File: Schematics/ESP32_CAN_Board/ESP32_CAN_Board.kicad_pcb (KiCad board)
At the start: 2 copper layers, 23 parts, among them J8 USB_C_Receptacle, U1 SN65HVD230, U7 LDL1117-3.3

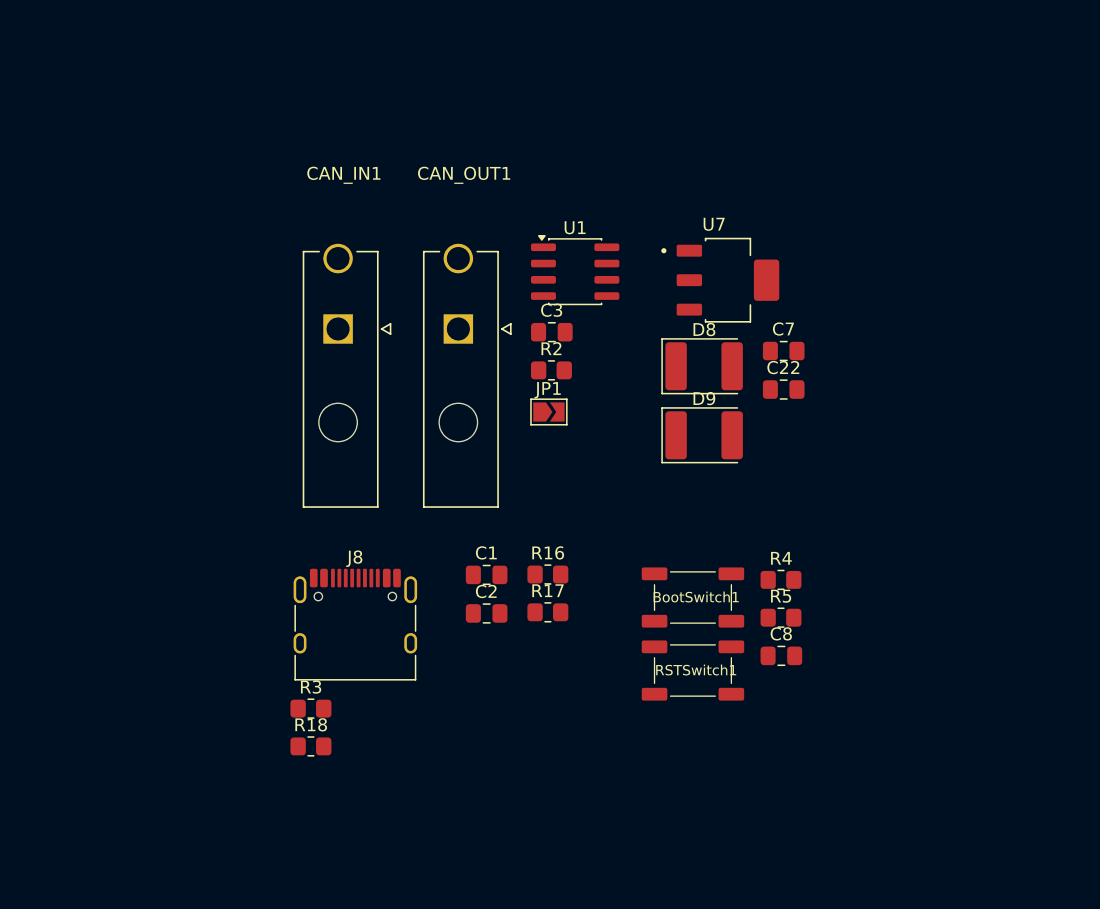
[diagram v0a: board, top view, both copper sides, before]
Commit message: initial design completed
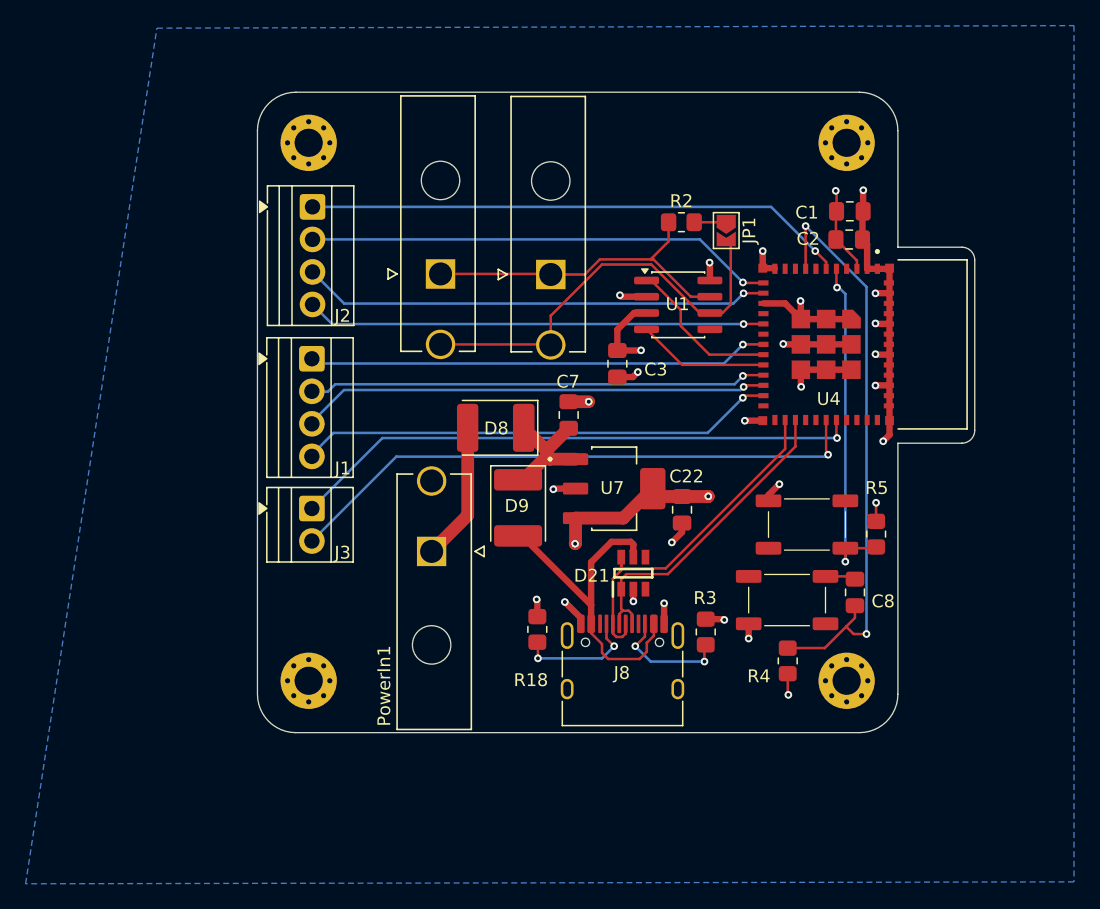
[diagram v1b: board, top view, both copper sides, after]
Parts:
- removed R16, R17: 10k, Resistor_SMD:R_0805_2012Metric_Pad1.20x1.40mm_HandSolder
- added D21: SRV05-4.TCT, myFootprints:SOT95P280X145-6N, F.Cu at (129.3, 87.5)
- added J1: Screw_Terminal_01x04, TerminalBlock:TerminalBlock_Xinya_XY308-2.54-4P_1x04_P2.54mm_Horizontal, F.Cu at (104.2, 70.8)
- added J2: Screw_Terminal_01x04, TerminalBlock:TerminalBlock_Xinya_XY308-2.54-4P_1x04_P2.54mm_Horizontal, F.Cu at (104.3, 59.0)
- added J3: Screw_Terminal_01x02, TerminalBlock:TerminalBlock_Xinya_XY308-2.54-2P_1x02_P2.54mm_Horizontal, F.Cu at (104.2, 82.5)
- added PowerIn1: 2 pin Molex, myFootprints:MOLEX_26013114, F.Cu at (113.6, 85.8)
- added REF**: MountingHole_2.2mm_M2_Pad_Via, MountingHole:MountingHole_2.2mm_M2_Pad_Via, F.Cu at (146.0, 96.0)
- added REF**: MountingHole_2.2mm_M2_Pad_Via, MountingHole:MountingHole_2.2mm_M2_Pad_Via, F.Cu at (104.0, 96.0)
- added REF**: MountingHole_2.2mm_M2_Pad_Via, MountingHole:MountingHole_2.2mm_M2_Pad_Via, F.Cu at (146.0, 54.0)
- added REF**: MountingHole_2.2mm_M2_Pad_Via, MountingHole:MountingHole_2.2mm_M2_Pad_Via, F.Cu at (104.0, 54.0)
- added U4: ESP32-C3-MINI-1-N4, myFootprints:XCVR_ESP32-C3-MINI-1-N4, F.Cu at (147.1, 69.7)
- moved C2 40.7 mm to (146.2, 61.5)
- moved C1 40.1 mm to (146.2, 59.3)
- moved R3 31.4 mm to (135.0, 92.1), turned to 90 degrees
- moved J8 21.2 mm to (128.5, 95.5)
- moved R18 19.9 mm to (121.8, 91.9), turned to 90 degrees
- moved JP1 19.8 mm to (136.6, 60.8), turned to -90 degrees
- moved U7 18.5 mm to (127.8, 81.0)
- moved C7 17.5 mm to (124.3, 75.2), turned to 90 degrees
- moved D8 17.0 mm to (118.6, 76.2), turned to 180 degrees
- moved D9 15.6 mm to (120.3, 82.5), turned to -90 degrees
- moved R2 15.4 mm to (133.1, 60.1)
- moved C22 12.3 mm to (133.2, 82.6), turned to -90 degrees
- moved BootSwitch1 10.6 mm to (142.9, 83.8)
- moved R5 9.88 mm to (148.3, 84.5), turned to -90 degrees
- moved RSTSwitch1 9.18 mm to (141.3, 89.7)
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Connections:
- C1 pad 1: /MCU/ESPPower -> +3.3V
- C2 pad 1: /MCU/ESPPower -> +3.3V
- C22 pad 1: /MCU/ESPPower -> +3.3V
- U7 pad 3: /MCU/ESPPower -> +3.3V
- U7 pad 4: /MCU/ESPPower -> +3.3V
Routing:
- net GND: track 0.00 -> 69.9 mm, vias 0 -> 24
- net /MCU/NRST: track 0.00 -> 46.2 mm, vias 0 -> 2
- net Net-(J3-Pin_2): track 0.00 -> 45.9 mm, vias 0 -> 1
- net Net-(J3-Pin_1): track 0.00 -> 44.7 mm, vias 0 -> 1
- net /MCU/Pin6: track 0.00 -> 42.4 mm, vias 0 -> 1
- net Net-(J1-Pin_4): track 0.00 -> 37.4 mm, vias 0 -> 1
- net Net-(J1-Pin_3): track 0.00 -> 36.7 mm, vias 0 -> 1
- net /MCU/Pin12: track 0.00 -> 36.6 mm, vias 0 -> 1
- net /MCU/Pin13: track 0.00 -> 36.6 mm, vias 0 -> 1
- net /MCU/Pin18: track 0.00 -> 36.2 mm, vias 0 -> 1
- net Net-(J1-Pin_2): track 0.00 -> 36.0 mm, vias 0 -> 1
- net /MCU/Pin16: track 0.00 -> 35.8 mm, vias 0 -> 1
- net /CAN/CANL: track 0.00 -> 33.7 mm
- net +3.3V: track 0.00 -> 29.0 mm, vias 0 -> 6
- net /MCU/D-: track 0.00 -> 28.0 mm
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- added copper zone on In2.Cu, net +3.3V
- added copper zone on B.Cu, net GND
- added copper zone on In1.Cu, net GND
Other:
- board outline added: 56 x 50 mm
- copper layers 2 -> 4
